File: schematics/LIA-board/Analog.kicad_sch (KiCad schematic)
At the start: 0 parts

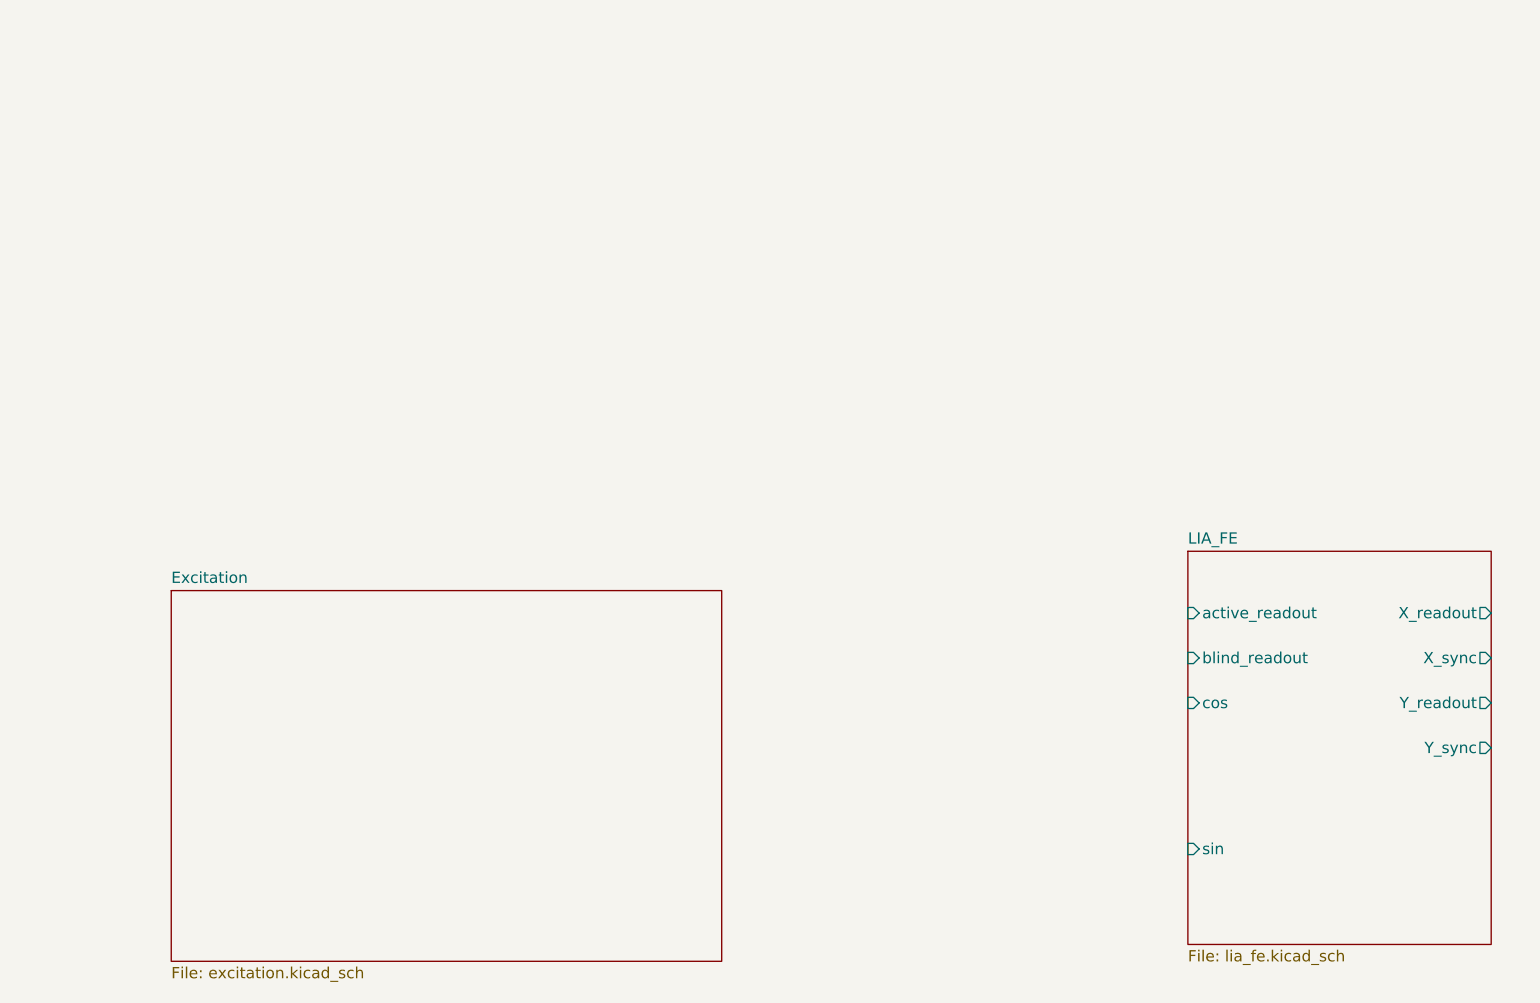
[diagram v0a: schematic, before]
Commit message: commit before changing LIA
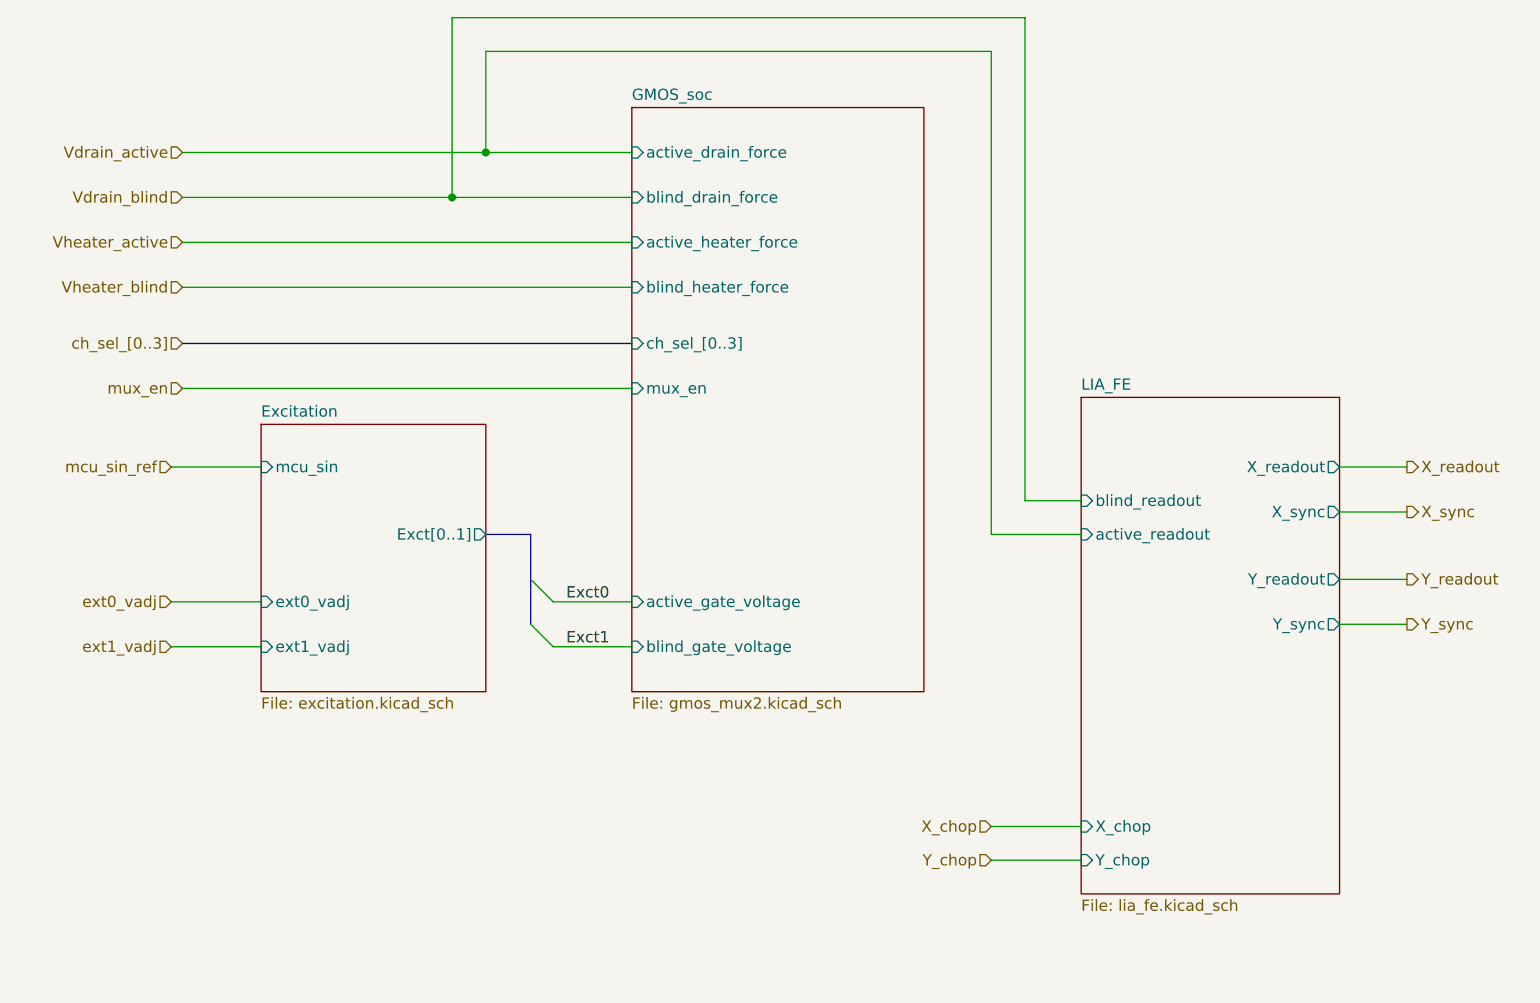
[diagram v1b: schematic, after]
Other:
- added sheet GMOS_soc (gmos_mux2.kicad_sch)
- sheet Excitation ports: added Exct[0..1], ext0_vadj, ext1_vadj, mcu_sin; removed none
- sheet LIA_FE ports: added X_chop, Y_chop; removed cos, sin
